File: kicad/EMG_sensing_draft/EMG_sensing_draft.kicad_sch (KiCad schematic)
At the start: 74 parts, among them J1 USB_A_0480370001, J2 EMG_SIGNAL, J3 DEBUG, U11 MCP1702T-3302E_CB, U13 Opamp_MCP6024T-E/ST, U14 MCP6021, U2 MCP6N11-002E/SN, U3 W25Q128JV, U5 ISL90462WIH627Z-TKCT-ND, U6 RP2040, U9 RN4871-I/RM140, Y1 12MHz

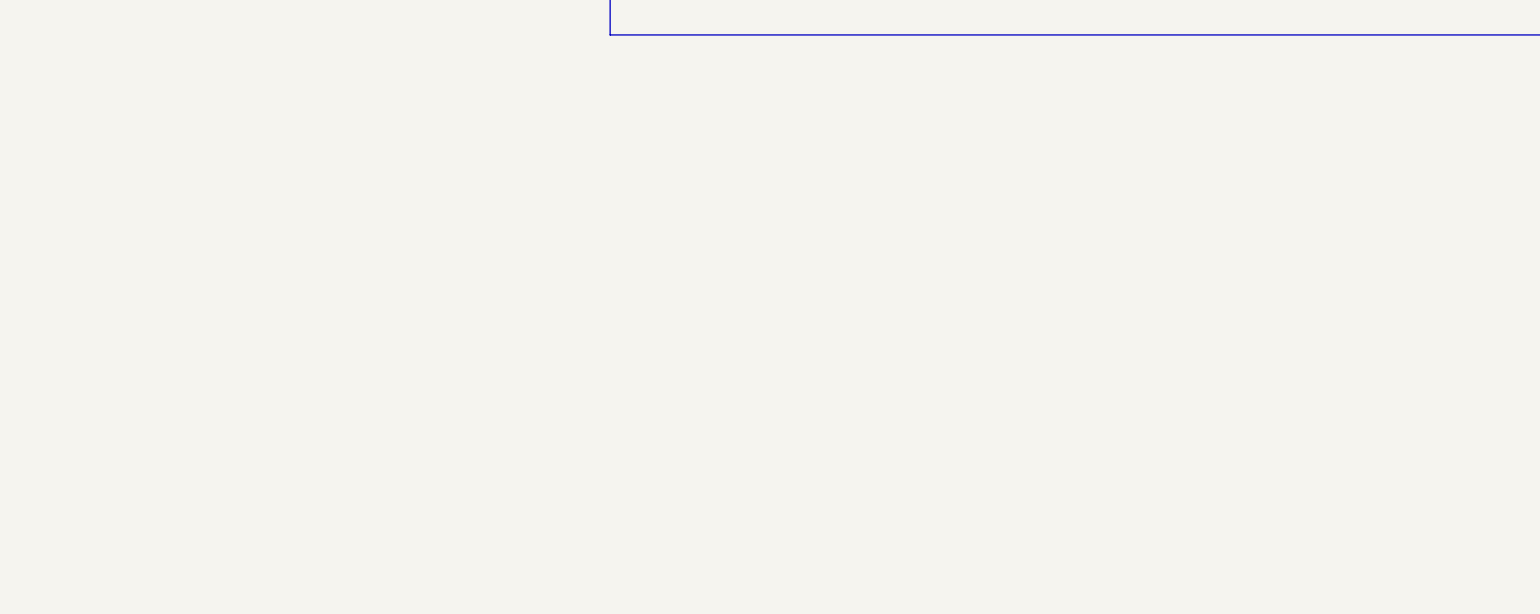
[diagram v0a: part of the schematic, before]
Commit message: adde reformmated filtering symbol
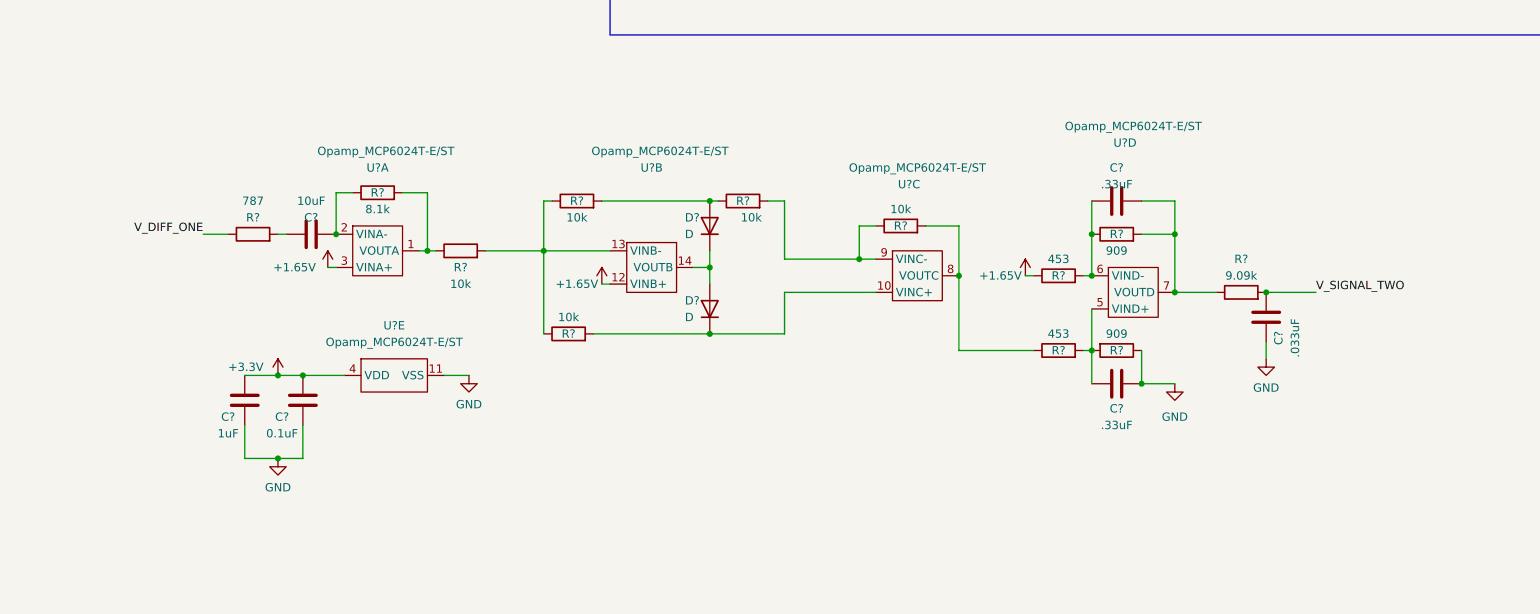
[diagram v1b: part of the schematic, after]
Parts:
- added C? (x2): .33uF, Capacitor_SMD:C_0603_1608Metric, symbol Device:C
- added C?: 1uF, Capacitor_SMD:C_0603_1608Metric, symbol Device:C
- added C?: 0.1uF, Capacitor_SMD:C_0603_1608Metric, symbol Device:C
- added C?: .033uF, Capacitor_SMD:C_0603_1608Metric, symbol Device:C
- added C?: 10uF, Capacitor_SMD:C_0603_1608Metric, symbol Device:C
- added D? (x2): D, Diode_SMD:D_0805_2012Metric, symbol Device:D
- added R?: 787, Resistor_SMD:R_0603_1608Metric, symbol Device:R
- added R? (x2): 453, Resistor_SMD:R_0603_1608Metric, symbol Device:R
- added R?: 9.09k, Resistor_SMD:R_0603_1608Metric, symbol Device:R
- added R? (x5): 10k, Resistor_SMD:R_0603_1608Metric, symbol Device:R
- added R? (x2): 909, Resistor_SMD:R_0603_1608Metric, symbol Device:R
- added R?: 8.1k, Resistor_SMD:R_0603_1608Metric, symbol Device:R
- added U? (x5): Opamp_MCP6024T-E/ST, MCP6024:MCP6024T, symbol Device:Opamp_MCP6024T-E/ST
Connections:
- net +1.65V: now also R?.1, U?.12 (VINB+), U?.3 (VINA+)
- net +3.3V: now also C?.2, C?.2, U?.4 (VDD)
- net GND: now also C?.1, C?.1, C?.1, C?.2, R?.1, U?.11 (VSS)
- new net: C?.2, R?.2, R?.2, U?.5 (VIND+)
- new net: C?.1, R?.1, R?.2, U?.6 (VIND-)
- new net: C?.2, R?.1, R?.2, U?.7 (VOUTD)
- new net: D?.1 (K), D?.2 (A), U?.14 (VOUTB)
- new net: D?.2 (A), R?.1, R?.2
- new net: D?.1 (K), R?.2, U?.10 (VINC+)
- new net: R?.1, R?.1, R?.2, U?.13 (VINB-)
- new net: C?.1, R?.2
- new net: R?.1, R?.2, U?.8 (VOUTC)
- new net: R?.1, R?.2, U?.9 (VINC-)
- new net: R?.1, R?.2, U?.1 (VOUTA)
- new net: C?.2, R?.1, U?.2 (VINA-)
- new net V_DIFF_ONE: R?.1
- new net V_SIGNAL_TWO: C?.1, R?.2
